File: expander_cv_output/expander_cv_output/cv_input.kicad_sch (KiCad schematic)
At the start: 6 parts

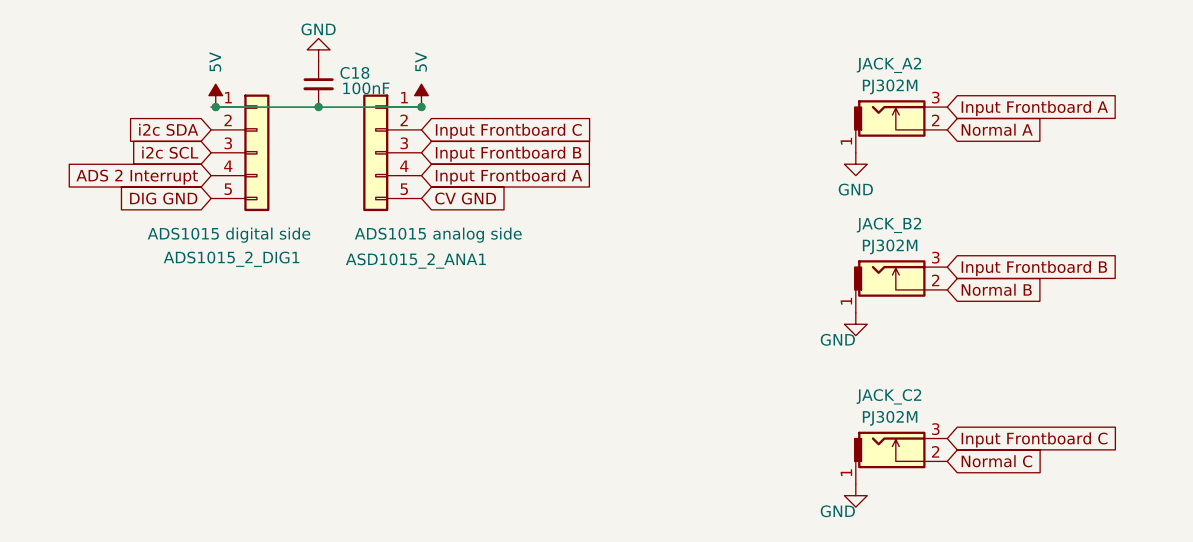
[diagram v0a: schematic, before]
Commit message: fixed incorrectly reversed analog input pins *facepalm*
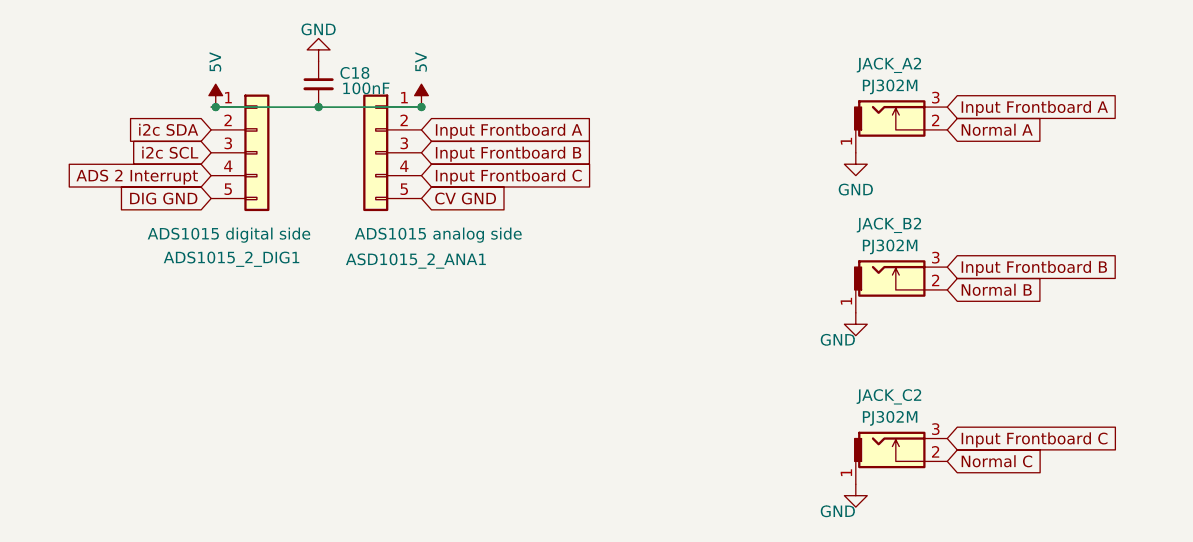
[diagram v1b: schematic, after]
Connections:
- net Input Frontboard A: now also ASD1015_2_ANA1.2 (Pin_2); no longer ASD1015_2_ANA1.4 (Pin_4)
- net Input Frontboard C: now also ASD1015_2_ANA1.4 (Pin_4); no longer ASD1015_2_ANA1.2 (Pin_2)
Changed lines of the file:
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@@
 	(global_label "Input Frontboard A"
 		(shape input)
+		(at 80.01 30.48 0)
+		(fields_autoplaced yes)
+		(effects
+			(font
+				(size 1.27 1.27)
+			)
+			(justify left)
+		)
+		(property "Intersheetrefs" "${INTERSHEET_REFS}"
+			(at 101.0772 30.48 0)
+			(effects
+				(font
+					(size 1.27 1.27)
+				)
+				(justify left)
+				(hide yes)
+			)
+		)
+	)
+	(global_label "Input Frontboard B"
+		(shape input)
+		(at 138.43 45.72 0)
+		(fields_autoplaced yes)
+		(effects
+			(font
+				(size 1.27 1.27)
+			)
+			(justify left)
+		)
+		(property "Intersheetrefs" "${INTERSHEET_REFS}"
+			(at 159.6786 45.72 0)
+			(effects
+				(font
+					(size 1.27 1.27)
+				)
+				(justify left)
+				(hide yes)
+			)
+		)
+	)
+	(global_label "i2c SCL"
+		(shape input)
+		(at 56.642 33.02 180)
+		(fields_autoplaced yes)
+		(effects
+			(font
+				(size 1.27 1.27)
+			)
+			(justify right)
+		)
+		(property "Intersheetrefs" "${INTERSHEET_REFS}"
+			(at 47.2179 33.02 0)
+			(effects
+				(font
+					(size 1.27 1.27)
+				)
+				(justify right)
+				(hide yes)
+			)
+		)
+	)
+	(global_label "Normal C"
+		(shape input)
+		(at 138.43 67.31 0)
+		(fields_autoplaced yes)
+		(effects
+			(font
+				(size 1.27 1.27)
+			)
+			(justify left)
+		)
+		(property "Intersheetrefs" "${INTERSHEET_REFS}"
+			(at 150.426 67.31 0)
+			(effects
+				(font
+					(size 1.27 1.27)
+				)
+				(justify left)
+				(hide yes)
+			)
+		)
+	)
+	(global_label "Input Frontboard C"
+		(shape input)
+		(at 138.43 64.77 0)
+		(fields_autoplaced yes)
+		(effects
+			(font
+				(size 1.27 1.27)
+			)
+			(justify left)
+		)
+		(property "Intersheetrefs" "${INTERSHEET_REFS}"
+			(at 159.6786 64.77 0)
+			(effects
+				(font
+					(size 1.27 1.27)
+				)
+				(justify left)
+				(hide yes)
+			)
+		)
+	)
+	(global_label "Normal A"
+		(shape input)
+		(at 138.43 30.48 0)
+		(fields_autoplaced yes)
+		(effects
+			(font
+				(size 1.27 1.27)
+			)
+			(justify left)
+		)
+		(property "Intersheetrefs" "${INTERSHEET_REFS}"
+			(at 150.2446 30.48 0)
+			(effects
+				(font
+					(size 1.27 1.27)
+				)
+				(justify left)
+				(hide yes)
+			)
+		)
+	)
+	(global_label "Input Frontboard A"
+		(shape input)
+		(at 138.43 27.94 0)
+		(fields_autoplaced yes)
+		(effects
+			(font
+				(size 1.27 1.27)
+			)
+			(justify left)
+		)
+		(property "Intersheetrefs" "${INTERSHEET_REFS}"
+			(at 159.4972 27.94 0)
+			(effects
+				(font
+					(size 1.27 1.27)
+				)
+				(justify left)
+				(hide yes)
+			)
+		)
+	)
+	(global_label "DIG GND"
+		(shape input)
+		(at 56.642 38.1 180)
+		(fields_autoplaced yes)
+		(effects
+			(font
+				(size 1.27 1.27)
+			)
+			(justify right)
+		)
+		(property "Intersheetrefs" "${INTERSHEET_REFS}"
+			(at 45.9589 38.1 0)
+			(effects
+				(font
+					(size 1.27 1.27)
+				)
+				(justify right)
+				(hide yes)
+			)
+		)
+	)
+	(global_label "ADS 2 Interrupt"
+		(shape input)
+		(at 56.642 35.56 180)
+		(fields_autoplaced yes)
+		(effects
+			(font
+				(size 1.27 1.27)
+			)
+			(justify right)
+		)
+		(property "Intersheetrefs" "${INTERSHEET_REFS}"
+			(at 38.8592 35.56 0)
+			(effects
+				(font
+					(size 1.27 1.27)
+				)
+				(justify right)
+				(hide yes)
+			)
+		)
+	)
+	(global_label "Input Frontboard C"
+		(shape input)
 		(at 80.01 35.56 0)
 		(fields_autoplaced yes)
@@
 		)
 		(property "Intersheetrefs" "${INTERSHEET_REFS}"
-			(at 101.0772 35.56 0)
-			(effects
-				(font
-					(size 1.27 1.27)
-				)
-				(justify left)
-				(hide yes)
-			)
-		)
-	)
-	(global_label "Input Frontboard B"
-		(shape input)
-		(at 138.43 45.72 0)
-		(fields_autoplaced yes)
-		(effects
-			(font
-				(size 1.27 1.27)
-			)
-			(justify left)
-		)
-		(property "Intersheetrefs" "${INTERSHEET_REFS}"
-			(at 159.6786 45.72 0)
-			(effects
-				(font
-					(size 1.27 1.27)
-				)
-				(justify left)
-				(hide yes)
-			)
-		)
-	)
-	(global_label "i2c SCL"
-		(shape input)
-		(at 56.642 33.02 180)
-		(fields_autoplaced yes)
-		(effects
-			(font
-				(size 1.27 1.27)
-			)
-			(justify right)
-		)
-		(property "Intersheetrefs" "${INTERSHEET_REFS}"
-			(at 47.2179 33.02 0)
-			(effects
-				(font
-					(size 1.27 1.27)
-				)
-				(justify right)
-				(hide yes)
-			)
-		)
-	)
-	(global_label "Normal C"
-		(shape input)
-		(at 138.43 67.31 0)
-		(fields_autoplaced yes)
-		(effects
-			(font
-				(size 1.27 1.27)
-			)
-			(justify left)
-		)
-		(property "Intersheetrefs" "${INTERSHEET_REFS}"
-			(at 150.426 67.31 0)
-			(effects
-				(font
-					(size 1.27 1.27)
-				)
-				(justify left)
-				(hide yes)
-			)
-		)
-	)
-	(global_label "Input Frontboard C"
-		(shape input)
-		(at 138.43 64.77 0)
-		(fields_autoplaced yes)
-		(effects
-			(font
-				(size 1.27 1.27)
-			)
-			(justify left)
-		)
-		(property "Intersheetrefs" "${INTERSHEET_REFS}"
-			(at 159.6786 64.77 0)
-			(effects
-				(font
-					(size 1.27 1.27)
-				)
-				(justify left)
-				(hide yes)
-			)
-		)
-	)
-	(global_label "Normal A"
-		(shape input)
-		(at 138.43 30.48 0)
-		(fields_autoplaced yes)
-		(effects
-			(font
-				(size 1.27 1.27)
-			)
-			(justify left)
-		)
-		(property "Intersheetrefs" "${INTERSHEET_REFS}"
-			(at 150.2446 30.48 0)
-			(effects
-				(font
-					(size 1.27 1.27)
-				)
-				(justify left)
-				(hide yes)
-			)
-		)
-	)
-	(global_label "Input Frontboard A"
-		(shape input)
-		(at 138.43 27.94 0)
-		(fields_autoplaced yes)
-		(effects
-			(font
-				(size 1.27 1.27)
-			)
-			(justify left)
-		)
-		(property "Intersheetrefs" "${INTERSHEET_REFS}"
-			(at 159.4972 27.94 0)
-			(effects
-				(font
-					(size 1.27 1.27)
-				)
-				(justify left)
-				(hide yes)
-			)
-		)
-	)
-	(global_label "DIG GND"
-		(shape input)
-		(at 56.642 38.1 180)
-		(fields_autoplaced yes)
-		(effects
-			(font
-				(size 1.27 1.27)
-			)
-			(justify right)
-		)
-		(property "Intersheetrefs" "${INTERSHEET_REFS}"
-			(at 45.9589 38.1 0)
-			(effects
-				(font
-					(size 1.27 1.27)
-				)
-				(justify right)
-				(hide yes)
-			)
-		)
-	)
-	(global_label "ADS 2 Interrupt"
-		(shape input)
-		(at 56.642 35.56 180)
-		(fields_autoplaced yes)
-		(effects
-			(font
-				(size 1.27 1.27)
-			)
-			(justify right)
-		)
-		(property "Intersheetrefs" "${INTERSHEET_REFS}"
-			(at 38.8592 35.56 0)
-			(effects
-				(font
-					(size 1.27 1.27)
-				)
-				(justify right)
-				(hide yes)
-			)
-		)
-	)
-	(global_label "Input Frontboard C"
-		(shape input)
-		(at 80.01 30.48 0)
-		(fields_autoplaced yes)
-		(effects
-			(font
-				(size 1.27 1.27)
-			)
-			(justify left)
-		)
-		(property "Intersheetrefs" "${INTERSHEET_REFS}"
-			(at 101.2586 30.48 0)
-			(effects
-				(font
+			(at 101.2586 35.56 0)
+			(effects
+				(font
